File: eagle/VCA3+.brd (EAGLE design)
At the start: 100 x 80 mm, 51 parts, among them IC1 TL072P, IC2 TL072P, Q1 2N3906, T2 2N3904, T3 2N3904, T4 2N3904, T5 2N3904, T6 2N3904

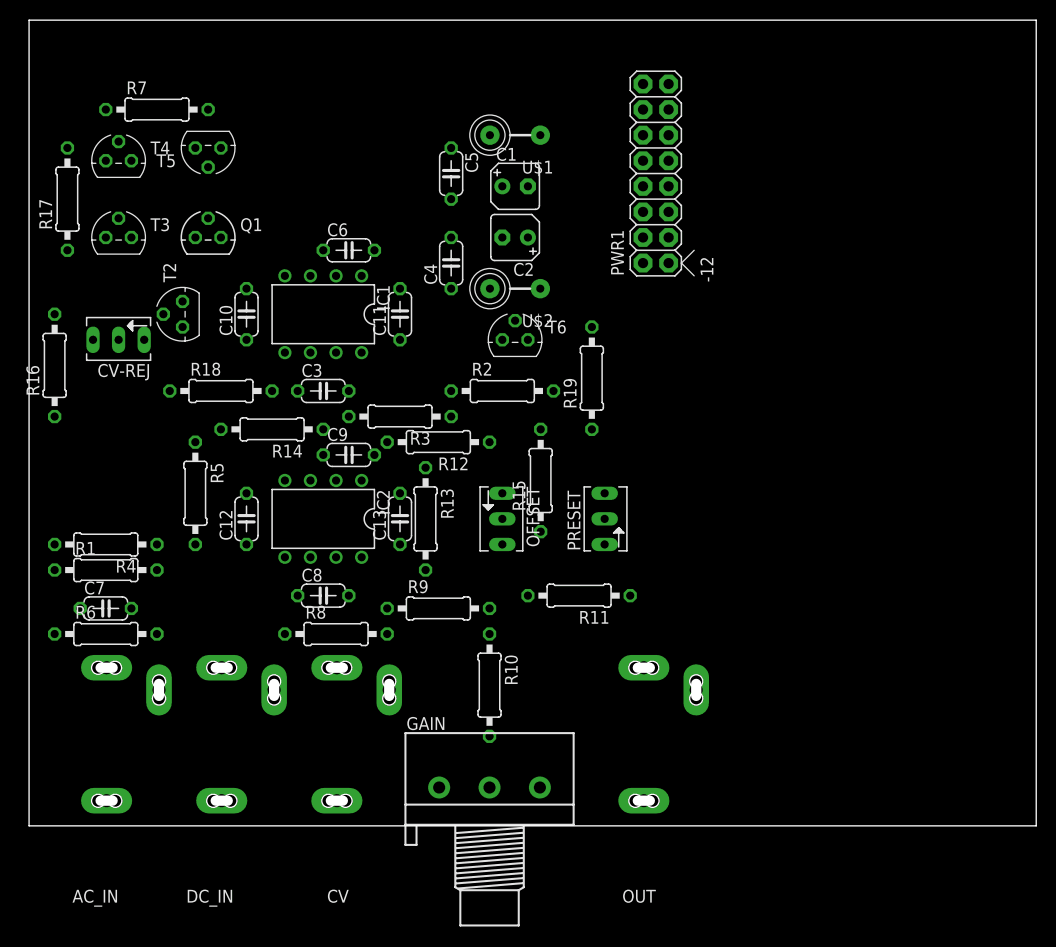
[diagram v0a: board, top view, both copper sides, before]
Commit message: close to layout
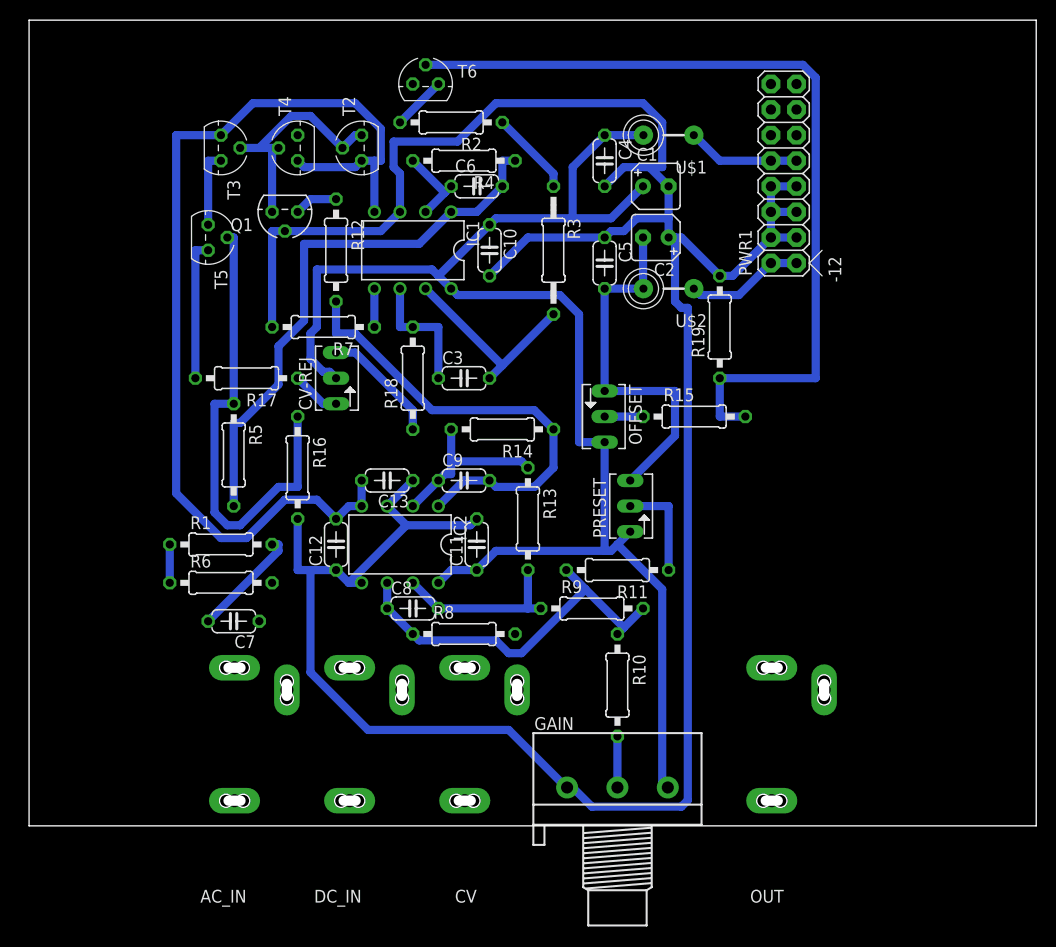
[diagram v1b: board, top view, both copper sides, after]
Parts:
- R3: device rcl:0207/10 -> rcl:0207/12
- moved R4 52.1 mm to (43.2, 66.0)
- moved R7 27.2 mm to (29.2, 49.5), turned to 180 degrees
- moved R2 27.1 mm to (41.9, 69.8), turned to 180 degrees
- moved T6 26.9 mm to (39.4, 73.7)
- moved R16 26.2 mm to (26.7, 35.6), turned to 270 degrees
- moved R17 25.1 mm to (21.6, 44.5), turned to 180 degrees
- moved C10 25.0 mm to (45.7, 57.1), turned to 270 degrees
- moved T2 24.3 mm to (33.0, 67.3)
- moved C11 24.1 mm to (44.5, 27.9)
- moved R14 22.9 mm to (47.0, 39.4)
- moved R3 22.5 mm to (52.1, 57.1), turned to 270 degrees
- moved CV-REJ 21.9 mm to (30.5, 44.5), turned to 90 degrees
- moved R12 21.6 mm to (30.5, 57.1), turned to 270 degrees
- moved R18 19.1 mm to (38.1, 44.5), turned to 90 degrees
- moved C4 18.3 mm to (57.1, 66.0), turned to 270 degrees
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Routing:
- net GND: track 0.00 -> 267.9 mm
- net +12V: track 0.00 -> 151.5 mm
- net -12V: track 0.00 -> 137.8 mm
- net N$24: track 0.00 -> 85.0 mm
- net N$8: track 0.00 -> 55.2 mm
- net N$22: track 0.00 -> 47.2 mm
- net N$18: track 0.00 -> 46.1 mm
- net N$11: track 0.00 -> 38.4 mm
- net N$19: track 0.00 -> 23.5 mm
- net N$5: track 0.00 -> 19.8 mm
- net N$25: track 0.00 -> 18.1 mm
- net N$9: track 0.00 -> 17.8 mm
- net N$15: track 0.00 -> 17.6 mm
- net N$17: track 0.00 -> 17.5 mm
- net N$27: track 0.00 -> 11.9 mm
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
